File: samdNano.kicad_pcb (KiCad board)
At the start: 2 copper layers, 43.2 x 17.8 mm, 6 parts, among them J1 Analog, J2 Digital

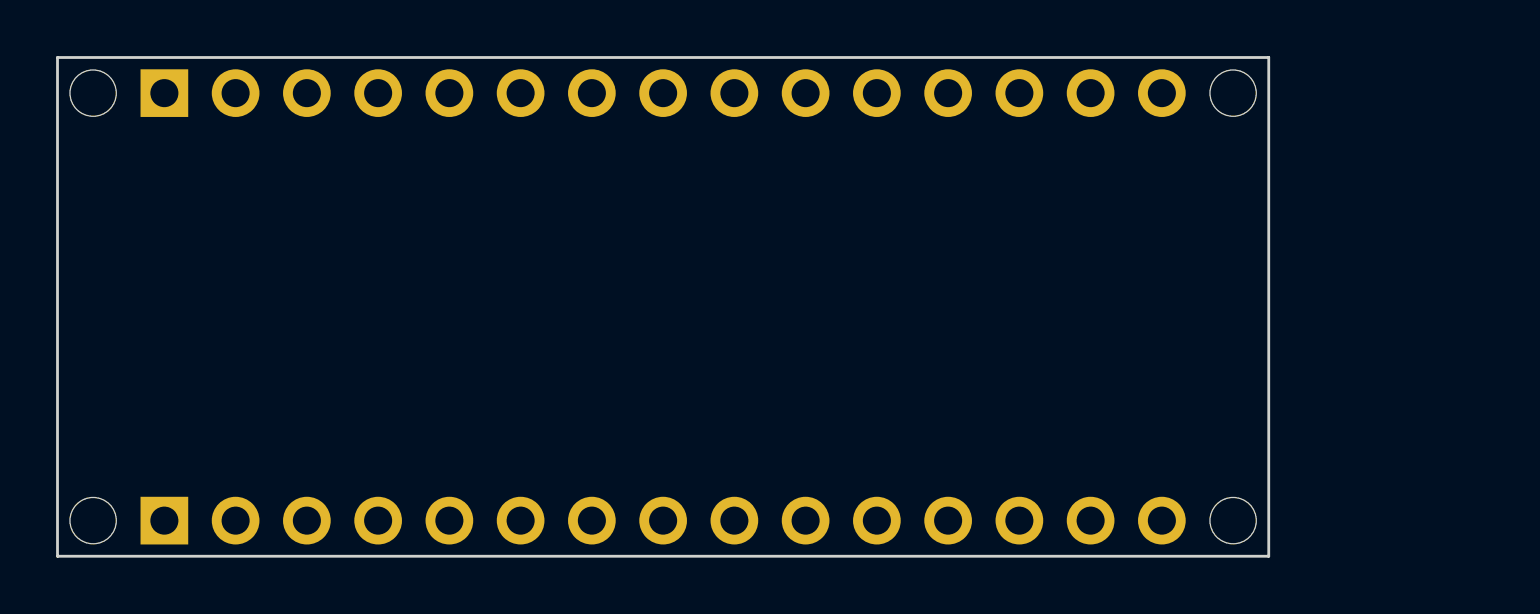
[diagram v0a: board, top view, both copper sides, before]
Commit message: Basic layout
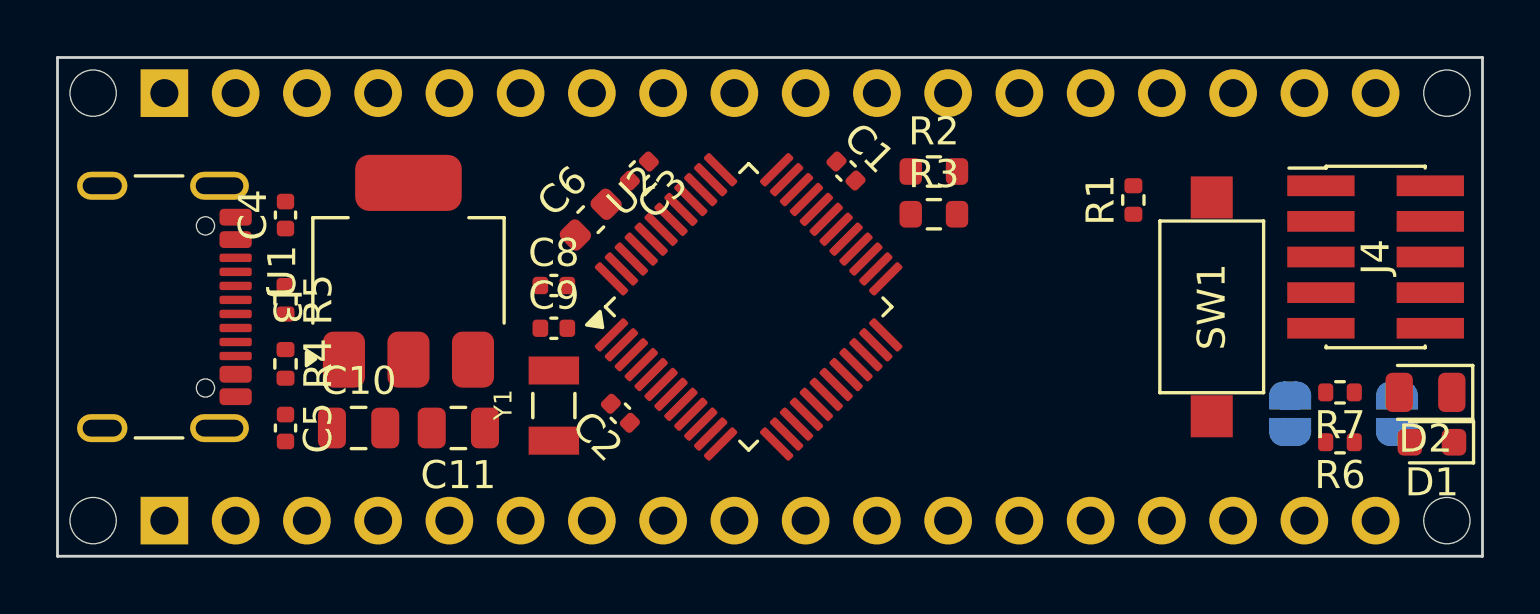
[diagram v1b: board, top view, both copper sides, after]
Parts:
- added C1: 100 nF, Capacitor_SMD:C_0402_1005Metric, F.Cu at (128.1, 86.3)
- added C10: 10 uF, Capacitor_SMD:C_0805_2012Metric, F.Cu at (110.7, 95.4)
- added C11: 10 uF, Capacitor_SMD:C_0805_2012Metric, F.Cu at (114.3, 95.4)
- added C2: 100 nF, Capacitor_SMD:C_0402_1005Metric, F.Cu at (120.1, 94.9)
- added C3: 100 nF, Capacitor_SMD:C_0402_1005Metric, F.Cu at (120.7, 86.3)
- added C4: 100 nF, Capacitor_SMD:C_0402_1005Metric, F.Cu at (108.1, 87.8)
- added C5: 100 nF, Capacitor_SMD:C_0402_1005Metric, F.Cu at (108.1, 95.4)
- added C6: 1 uF, Capacitor_SMD:C_0603_1608Metric, F.Cu at (119.0, 88.0)
- added C8: 22 pF, Capacitor_SMD:C_0402_1005Metric, F.Cu at (117.7, 90.3)
- added C9: 22 pF, Capacitor_SMD:C_0402_1005Metric, F.Cu at (117.7, 91.9)
- added D1: LED, LED_SMD:LED_0603_1608Metric, F.Cu at (149.0, 95.9)
- added D2: PWR_LED, LED_SMD:LED_0805_2012Metric, F.Cu at (148.8, 94.2)
- added J3: USB-C, Connector_USB:USB_C_Receptacle_GCT_USB4105-xx-A_16P_TopMnt_Horizontal, F.Cu at (102.7, 91.1)
- added J4: J Link, Connector_PinHeader_1.27mm:PinHeader_2x05_P1.27mm_Vertical_SMD, F.Cu at (147.0, 89.3)
- added JP3: LED_EN, Jumper:SolderJumper-2_P1.3mm_Open_RoundedPad1.0x1.5mm, B.Cu at (143.9, 94.9)
- added JP4: PWR_LED_EN, Jumper:SolderJumper-2_P1.3mm_Open_RoundedPad1.0x1.5mm, B.Cu at (147.8, 94.9)
- added R1: 220, Resistor_SMD:R_0402_1005Metric, F.Cu at (138.4, 87.3)
- added R2: 1.8 K, Resistor_SMD:R_0603_1608Metric, F.Cu at (131.2, 86.3)
- added R3: 1.8 K, Resistor_SMD:R_0603_1608Metric, F.Cu at (131.2, 87.8)
- added R4: 5.1 K, Resistor_SMD:R_0402_1005Metric, F.Cu at (108.1, 93.1)
- added R5: 5.1 K, Resistor_SMD:R_0402_1005Metric, F.Cu at (108.1, 90.9)
- added R6: 1 K, Resistor_SMD:R_0402_1005Metric, F.Cu at (145.7, 95.9)
- added R7: 1 K, Resistor_SMD:R_0402_1005Metric, F.Cu at (145.7, 94.2)
- added SW1: RESET, Button_Switch_SMD:SW_SPST_CK_RS282G05A3, F.Cu at (141.1, 91.1)
- added U1: AMS1117-3.3, Package_TO_SOT_SMD:SOT-223-3_TabPin2, F.Cu at (112.5, 89.8)
- added U2: ATSAMD21G18A-A, Package_QFP:TQFP-48_7x7mm_P0.5mm, F.Cu at (124.6, 91.1)
- added Y1: 32.768 kHz, CM7V-T1A-32.768K-12.5PF-20PPM-TA-QA:XTAL_CM7V-T1A-32.768K-12.5PF-20PPM-TA-QA, F.Cu at (117.7, 94.6)
- J1, J2: footprint Connector_PinHeader_2.54mm:PinHeader_1x15_P2.54mm_Vertical -> Connector_PinHeader_2.54mm:PinHeader_1x18_P2.54mm_Vertical
- moved MH3 7.62 mm to (149.5, 83.5)
- moved MH4 7.62 mm to (149.5, 98.7)
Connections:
- net /A4/SDA renamed A4
- net /A6 renamed A6
- net /A7 renamed A7
- net /D0/RX renamed DO
- net /~{RESET} renamed RST
- J1 pad 1: /D13/SCK -> D13
- J1 pad 3: /AREF -> AREF
- J1 pad 4: /A0 -> A0
- J1 pad 5: /A1 -> A1
- J1 pad 6: /A2 -> A2
- J1 pad 7: /A3 -> A3
- J1 pad 9: /A5/SCL -> A5
- J2 pad 1: /D12/MISO -> D12
- J2 pad 10: /*D3 -> D3
- J2 pad 11: /D2 -> D2
- J2 pad 15: /D1/TX -> D1
- J2 pad 2: /*D11/MOSI -> D11
- J2 pad 3: /*D10/SS -> D10
- J2 pad 4: /*D9 -> D9
- J2 pad 5: /D8 -> D8
- J2 pad 6: /D7 -> D7
- J2 pad 7: /*D6 -> D6
- J2 pad 8: /*D5 -> D5
- J2 pad 9: /D4 -> D4
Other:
- board size 43.2 x 17.8 mm -> 50.8 x 17.8 mm
- board text removed: "ICSP"
- board text removed: "USB Mini-B"
